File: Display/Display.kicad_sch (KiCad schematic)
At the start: 8 parts, among them Q1 ZXM61N03F, U1 E2206KS0E1

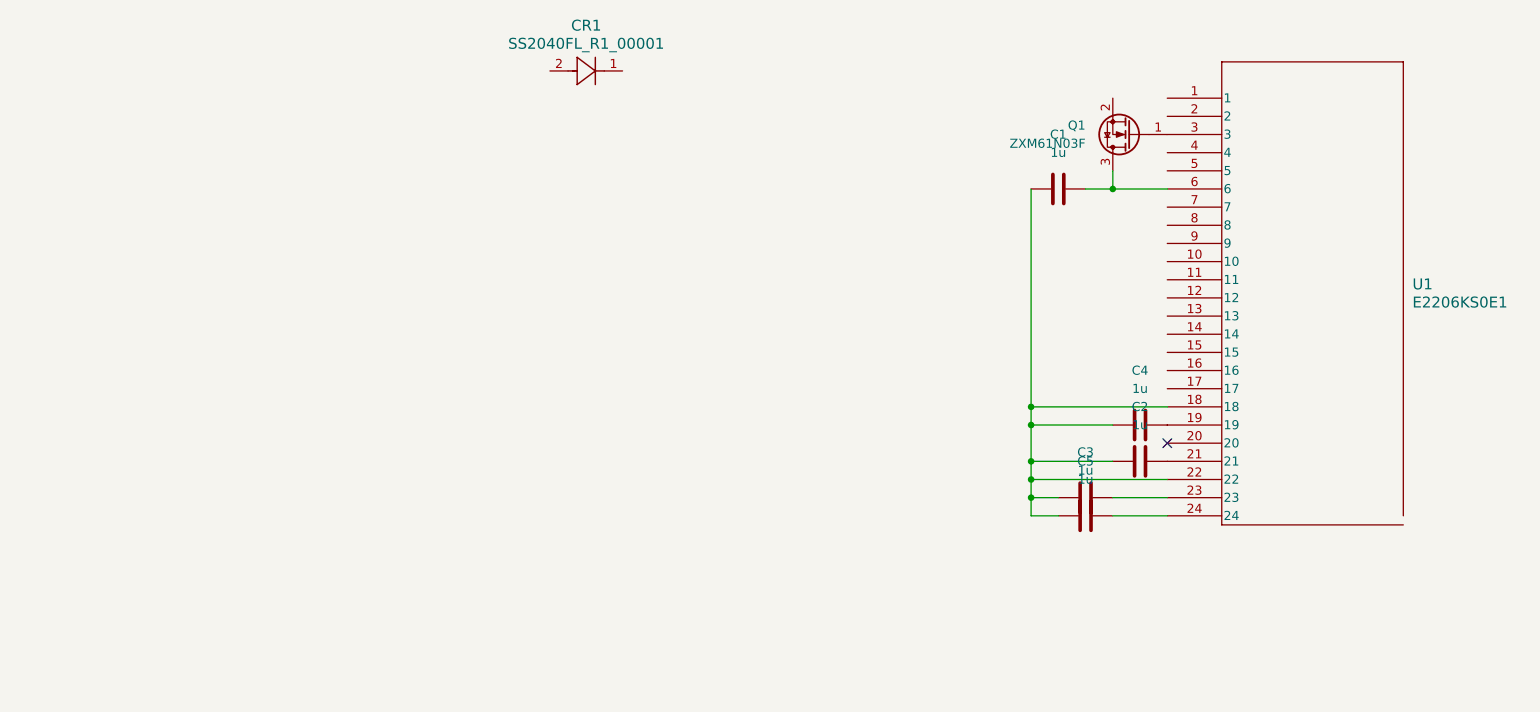
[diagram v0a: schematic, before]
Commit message: Oct11_Schematic
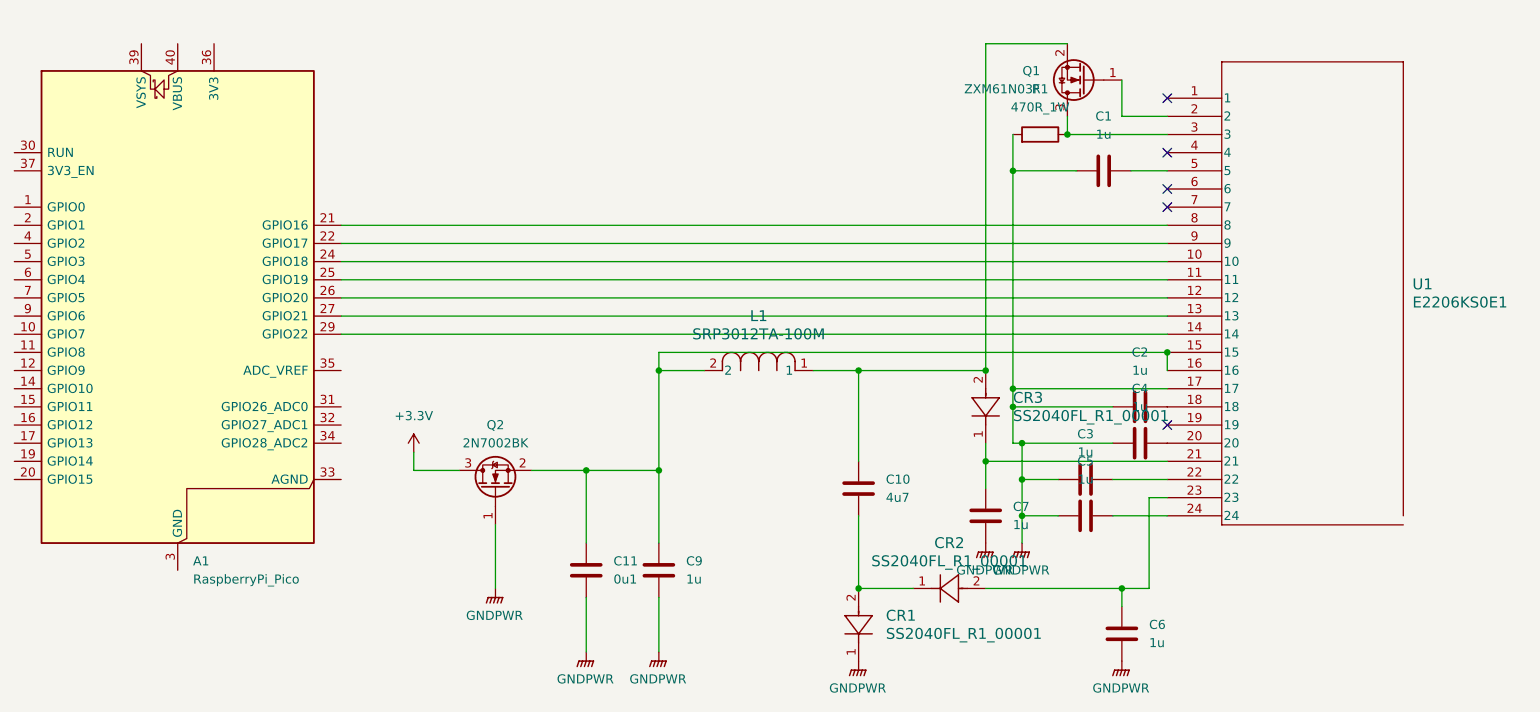
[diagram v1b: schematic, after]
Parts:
- added A1: RaspberryPi_Pico, Module:RaspberryPi_Pico_Common_Unspecified, symbol MCU_Module:RaspberryPi_Pico
- added C10: 4u7, rsx_capacitors:C_0805_2012Metric, symbol rsx_Capacitors:4u7
- added C11: 0u1, rsx_capacitors:C_0603_1608Metric, symbol rsx_Capacitors:0u1
- added C6, C7, C9: 1u, rsx_capacitors:C_0805_2012Metric, symbol rsx_Capacitors:1u
- added CR2, CR3: SS2040FL_R1_00001, CR_R1_00001_PNJ, symbol SS2040FL_R1_00001:SS2040FL_R1_00001
- added L1: SRP3012TA-100M, IND_SRP3012TA_BRN, symbol SRP3012TA-100M:SRP3012TA-100M
- added Q2: 2N7002BK, rsx_packages_TO_SOT:SOT-23, symbol rsx_Transistors:2N7002BK
- added R1: 470R_1W, rsx_resistors:R_2512_6332Metric, symbol rsx_Resistors:470R_1W
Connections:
- net at U1.10: now also A1.24 (GPIO18)
- net at U1.11: now also A1.25 (GPIO19)
- net at U1.12: now also A1.26 (GPIO20)
- net at U1.13: now also A1.27 (GPIO21)
- net at U1.14: now also A1.29 (GPIO22)
- net at U1.15: now also U1.16, C11.1, C9.2, L1.2, Q2.2 (S)
- net GNDPWR: now reaches U1.17
- net GNDPWR: now also C1.1, C2.1, C3.2, C4.1, C5.1, CR1.1, C11.2, C6.1, C7.1, C9.1, Q2.1 (G), R1.1
- net at U1.19: no longer C4.1
- net at U1.2: now also Q1.1 (G)
- net at U1.20: now also C4.2
- net at C2.2: now also U1.18; no longer U1.21
- net at C3.1: now also U1.22; no longer U1.23
- net at U1.3: now also Q1.3 (D), R1.2; no longer Q1.1 (G)
- net at U1.5: now also C1.2
- net at U1.8: now also A1.21 (GPIO16)
- net at U1.9: now also A1.22 (GPIO17)
- net at Q1.2 (S): now also C10.1, CR3.2, L1.1
- net at CR1.2: now also C10.2, CR2.1
- new net: C7.2, CR3.1, U1.21
- new net: C6.2, CR2.2, U1.23
- new net: A1.13 (GND), A1.18 (GND), A1.23 (GND), A1.28 (GND), A1.3 (GND), A1.38 (GND), A1.8 (GND)
- new net +3.3V: Q2.3 (D)
- now unconnected: U1.6
- no-connect marks 1 -> 5
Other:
- moved on the sheet: C2, C3, Q1
